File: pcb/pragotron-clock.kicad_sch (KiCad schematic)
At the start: 17 parts, among them J1 Conn_01x02, J2 Conn_01x03, J3 Conn_01x03, J4 Conn_01x02, J5 Conn_01x02, J6 Conn_01x04, U1 L293D

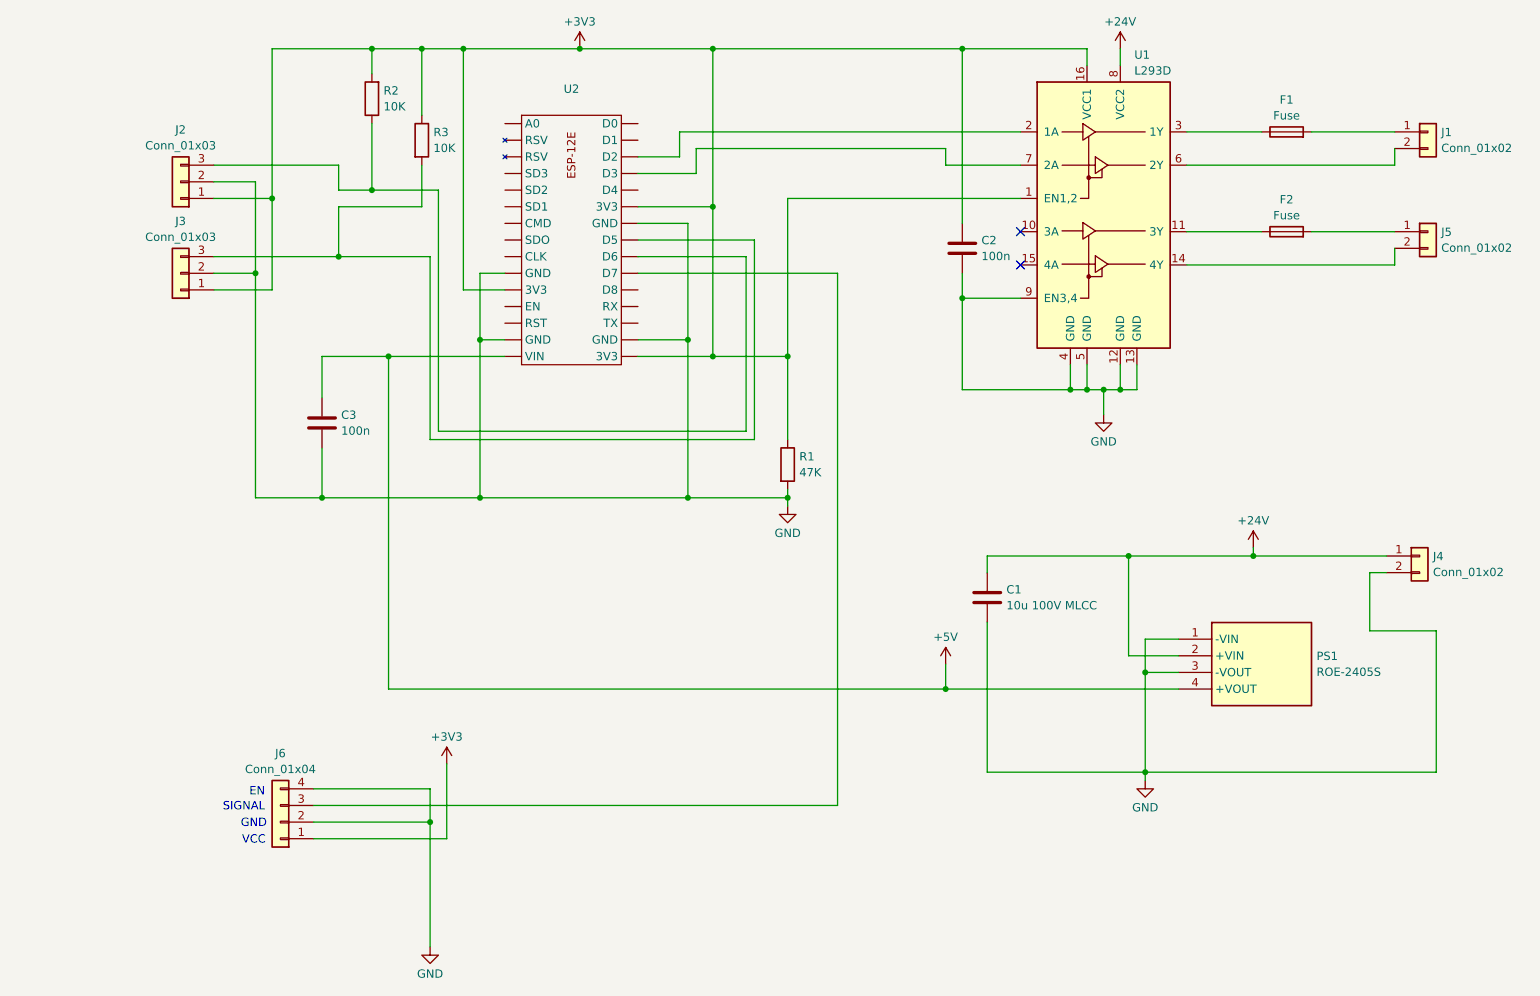
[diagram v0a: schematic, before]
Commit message: wip firmware and schematics
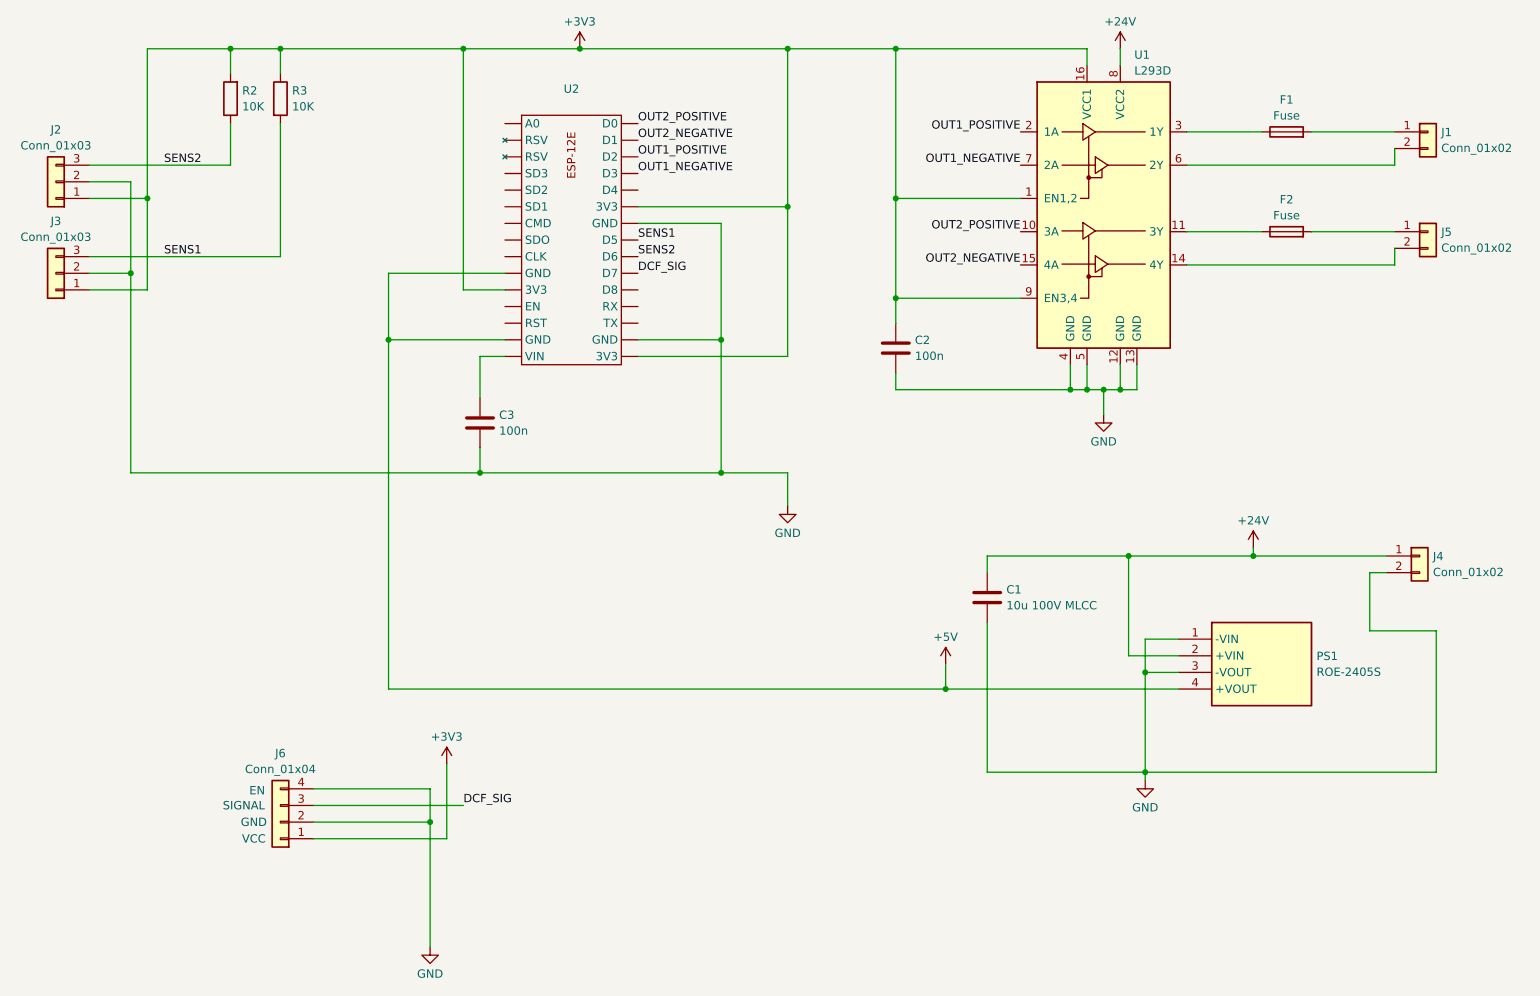
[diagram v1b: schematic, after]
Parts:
- removed R1: 47K, Resistor_THT:R_Axial_DIN0204_L3.6mm_D1.6mm_P7.62mm_Horizontal, symbol Device:R
- U2: value ~ -> (none)
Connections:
- net +3V3: now also U1.9 (EN3,4)
- net +5V: no longer C3.1
- net GND: no longer U1.9 (EN3,4)
- net OUT2_POSITIVE: now reaches U1.10 (3A)
- net OUT2_POSITIVE: now also U2. (3V3)
- net OUT2_NEGATIVE: now reaches U1.15 (4A)
- net OUT2_NEGATIVE: now also U2. (3V3)
- net OUT1_POSITIVE: now reaches U1.2 (1A), U2. (3V3)
- net OUT1_NEGATIVE: now reaches U1.7 (2A), U2. (3V3)
- net SENS1: now reaches J3.3 (Pin_3), R3.2, U2. (3V3)
- net DCF_SIG: now reaches J6.3 (Pin_3), U2. (3V3)
- net SENS2: now reaches J2.3 (Pin_3), R2.1, U2. (3V3)
- new net: C3.1, U2. (3V3)
- no-connect marks 2 -> 0
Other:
- moved on the sheet: C2, C3, J2, J3, R2, R3
